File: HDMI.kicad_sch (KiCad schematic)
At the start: 14 parts, among them IC8 TPS2557QDRBTQ1, J7 HDMI_A_1.4, U1 TPD1E05U06DYA

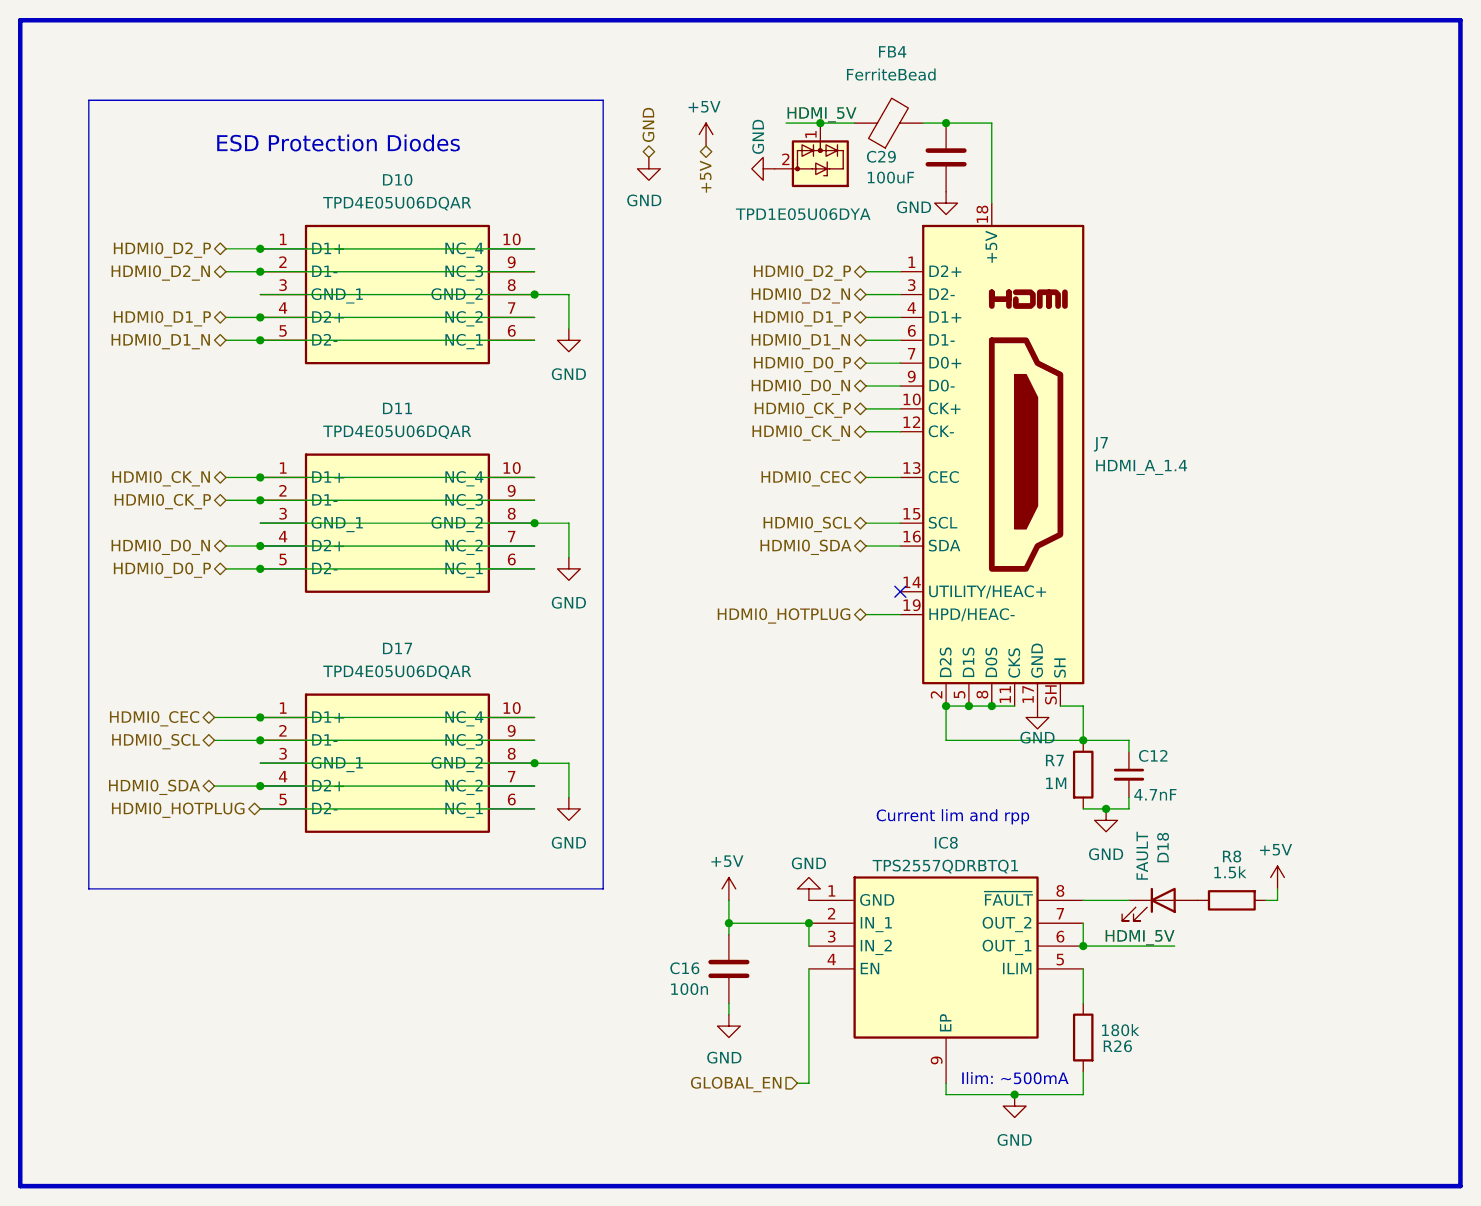
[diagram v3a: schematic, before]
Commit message: P/Ns
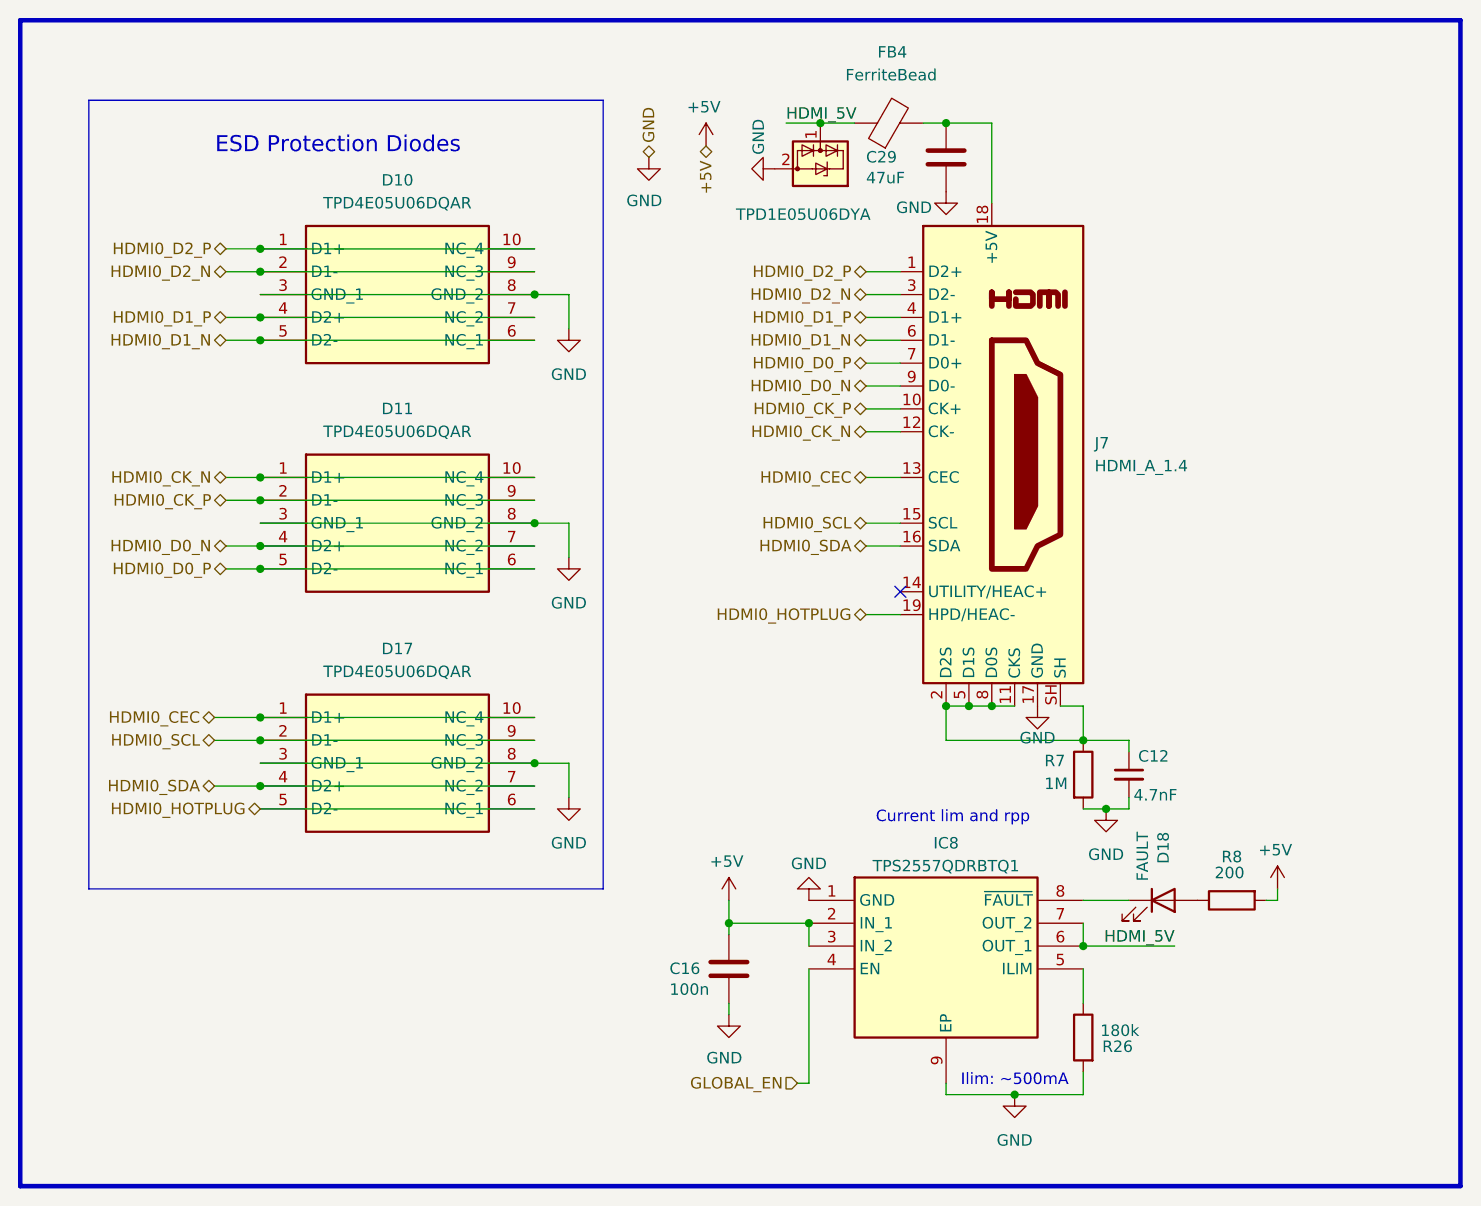
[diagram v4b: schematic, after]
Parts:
- C12: P/N (none) -> 06035C472K4T2A
- C16: P/N C0805C104M5RACTU -> MLASH168SB7104KTNA01
- C29: value 100uF -> 47uF; P/N C0805C104M5RACTU -> GRM21BR61A476ME15L
- D18: P/N APTD2012LCGCK -> LS Q976.01-N1Q2-1
- FB4: P/N BMC-Q2CY0220H -> BLM31PG121SN1L
- IC8: P/N (none) -> TPS2557QDRBTQ1
- J7: P/N (none) -> 2086581001
- R26: P/N (none) -> 560112116072
- R7: P/N (none) -> RCC06031M00FKEA
- R8: value 1.5k -> 200; P/N (none) -> SG73S1JTTD2000F
- U1: P/N (none) -> TPD1E05U06DYA
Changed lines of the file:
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@@
+			)
+		)
+		(property "Data" ""
+			(at 166.37 125.73 0)
+			(effects
+				(font
+					(size 1.27 1.27)
+				)
+				(hide yes)
+			)
+		)
+		(property "P/N" "TPS2557QDRBTQ1"
+			(at 166.37 125.73 0)
+			(effects
+				(font
+					(size 1.27 1.27)
+				)
+				(hide yes)
 			)
 		)
@@
 			)
 		)
-		(property "Value" "100uF"
+		(property "Value" "47uF"
 			(at 172.72 45.466 0)
 			(effects
@@
 			)
 		)
-		(property "P/N" "C0805C104M5RACTU"
+		(property "P/N" "GRM21BR61A476ME15L"
+			(at 181.61 43.18 0)
+			(effects
+				(font
+					(size 1.27 1.27)
+				)
+				(hide yes)
+			)
+		)
+		(property "Data" ""
 			(at 181.61 43.18 0)
 			(effects
@@
 			)
 		)
-		(property "Value" "1.5k"
+		(property "Value" "200"
 			(at 213.106 122.682 90)
 			(effects
@@
 			)
 		)
-		(property "P/N" ""
+		(property "P/N" "SG73S1JTTD2000F"
 			(at 213.36 125.73 0)
+			(effects
+				(font
+					(size 1.27 1.27)
+				)
+				(hide yes)
+			)
+		)
+		(property "Data" ""
+			(at 213.36 125.73 90)
 			(effects
 				(font
@@
 			)
 		)
-		(property "P/N" "APTD2012LCGCK"
+		(property "P/N" "LS Q976.01-N1Q2-1 "
 			(at 205.74 125.73 90)
 			(effects
@@
 			)
 		)
+		(property "Data" ""
+			(at 205.74 125.73 90)
+			(effects
+				(font
+					(size 1.27 1.27)
+				)
+				(hide yes)
+			)
+		)
 		(pin "1"
 		)
@@
 		)
 		(property "P/N" "TPD4E05U06DQAR"
+			(at 105.41 53.34 0)
+			(effects
+				(font
+					(size 1.27 1.27)
+				)
+				(hide yes)
+			)
+		)
+		(property "Data" ""
 			(at 105.41 53.34 0)
 			(effects
@@
 			)
 		)
-		(property "P/N" ""
+		(property "P/N" "560112116072"
+			(at 196.85 140.97 0)
+			(effects
+				(font
+					(size 1.27 1.27)
+				)
+				(hide yes)
+			)
+		)
+		(property "Data" ""
 			(at 196.85 140.97 0)
 			(effects
@@
 			)
 		)
-		(property "P/N" "BMC-Q2CY0220H "
+		(property "P/N" "BLM31PG121SN1L"
 			(at 175.26 39.37 0)
+			(effects
+				(font
+					(size 1.27 1.27)
+				)
+				(hide yes)
+			)
+		)
+		(property "Data" ""
+			(at 175.26 39.37 90)
 			(effects
 				(font
@@
 			)
 		)
+		(property "Data" ""
+			(at 201.93 111.76 0)
+			(effects
+				(font
+					(size 1.27 1.27)
+				)
+				(hide yes)
+			)
+		)
+		(property "P/N" "06035C472K4T2A"
+			(at 201.93 111.76 0)
+			(effects
+				(font
+					(size 1.27 1.27)
+				)
+				(hide yes)
+			)
+		)
 		(pin "1"
 		)
@@
 		(property "Description" "1-Channel ESD Protection for Super-Speed USB 3.0 Interface, SOD-523"
 			(at 167.64 44.45 0)
+			(effects
+				(font
+					(size 1.27 1.27)
+				)
+				(hide yes)
+			)
+		)
+		(property "Data" ""
+			(at 167.64 44.45 90)
+			(effects
+				(font
+					(size 1.27 1.27)
+				)
+				(hide yes)
+			)
+		)
+		(property "P/N" "TPD1E05U06DYA"
+			(at 167.64 44.45 90)
 			(effects
 				(font
@@
 			)
 		)
+		(property "Data" ""
+			(at 105.41 105.41 0)
+			(effects
+				(font
+					(size 1.27 1.27)
+				)
+				(hide yes)
+			)
+		)
 		(pin "5"
 		)
@@
 		)
 		(property "Description" "Resistor"
+			(at 196.85 111.76 0)
+			(effects
+				(font
+					(size 1.27 1.27)
+				)
+				(hide yes)
+			)
+		)
+		(property "Data" ""
+			(at 196.85 111.76 0)
+			(effects
+				(font
+					(size 1.27 1.27)
+				)
+				(hide yes)
+			)
+		)
+		(property "P/N" "RCC06031M00FKEA"
 			(at 196.85 111.76 0)
 			(effects
@@
 			)
 		)
+		(property "Data" ""
+			(at 105.41 78.74 0)
+			(effects
+				(font
+					(size 1.27 1.27)
+				)
+				(hide yes)
+			)
+		)
 		(pin "5"
 		)
@@
 			)
 		)
-		(property "P/N" "C0805C104M5RACTU"
+		(property "P/N" "MLASH168SB7104KTNA01 "
+			(at 157.48 133.35 0)
+			(effects
+				(font
+					(size 1.27 1.27)
+				)
+				(hide yes)
+			)
+		)
+		(property "Data" ""
 			(at 157.48 133.35 0)
 			(effects
@@
 			(at 186.69 76.2 0)
 			(effects
+				(font
+					(size 1.27 1.27)
+				)
+				(hide yes)
+			)
+		)
+		(property "Data" ""
+			(at 186.69 76.2 0)
+			(effects
+				(font
+					(size 1.27 1.27)
+				)
+				(hide yes)
+			)
+		)
+		(property "P/N" "2086581001"
+			(at 186.69 76.2 0)
+			(effects
